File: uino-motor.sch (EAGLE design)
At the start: 31 parts, among them J1 CON_TERMINAL_BLOCK_02-5MM, J2 CON_TERMINAL_BLOCK_02-5MM, J3 CON_TERMINAL_BLOCK_02-5MM, Q1 P-FET, U1 74*1G57, U2 74*1G57

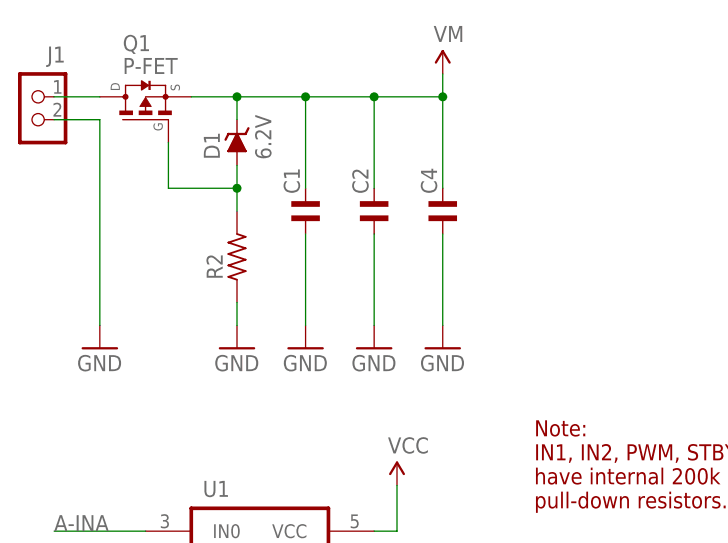
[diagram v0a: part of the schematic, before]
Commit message: Parts placed and major routing completed.
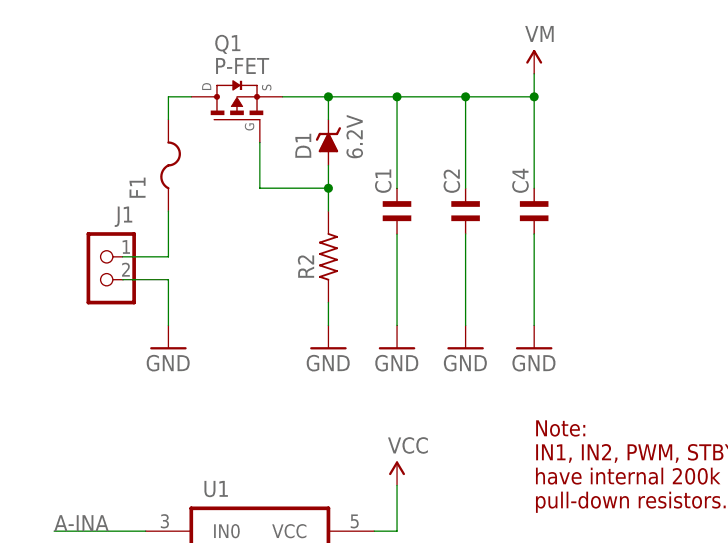
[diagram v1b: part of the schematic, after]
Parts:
- added F1: (no value), adi-misc:FUSE_PTC-TH
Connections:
- net N$10 renamed A01
- net N$11 renamed B01
- net N$12 renamed A02
- net N$13 renamed B02
- removed net N$8: J1.1, Q1.D
- new net N$5: F1.1, J1.1
- new net N$7: F1.2, Q1.D
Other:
- moved on the sheet: C1, C2, C4, D1, J1, Q1, R2
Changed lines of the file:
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@@
 <part name="R5" library="rc-master-smd" deviceset="R_" device="0805MP"/>
 <part name="GND15" library="SparkFun-Aesthetics" deviceset="GND" device=""/>
+<part name="F1" library="adi-misc" deviceset="FUSE_PTC" device="-TH"/>
 </parts>
 <sheets>
@@
 <instance part="J2" gate="CON" x="132.08" y="81.28" rot="MR180"/>
 <instance part="J3" gate="CON" x="132.08" y="60.96" rot="MR180"/>
-<instance part="J1" gate="CON" x="5.08" y="152.4" rot="MR0"/>
+<instance part="J1" gate="CON" x="12.7" y="134.62" rot="MR0"/>
 <instance part="GND8" gate="1" x="121.92" y="50.8"/>
 <instance part="GND3" gate="1" x="83.82" y="50.8"/>
@@
 <instance part="R1" gate="G$1" x="71.12" y="73.66"/>
 <instance part="SUPPLY3" gate="G$1" x="60.96" y="91.44"/>
-<instance part="Q1" gate="G$1" x="15.24" y="152.4" smashed="yes" rot="R90">
-<attribute name="VALUE" x="12.7" y="154.94" size="1.778" layer="96"/>
-<attribute name="NAME" x="12.7" y="157.48" size="1.778" layer="95"/>
+<instance part="Q1" gate="G$1" x="25.4" y="152.4" smashed="yes" rot="R90">
+<attribute name="VALUE" x="22.86" y="154.94" size="1.778" layer="96"/>
+<attribute name="NAME" x="22.86" y="157.48" size="1.778" layer="95"/>
 </instance>
-<instance part="D1" gate="G$1" x="25.4" y="147.32" rot="R90"/>
-<instance part="R2" gate="G$1" x="25.4" y="134.62" rot="R90"/>
-<instance part="GND5" gate="1" x="25.4" y="124.46"/>
-<instance part="SUPPLY6" gate="VDD" x="48.26" y="154.94"/>
-<instance part="C1" gate="G$1" x="33.02" y="139.7" rot="R90"/>
-<instance part="C2" gate="G$1" x="40.64" y="139.7" rot="R90"/>
-<instance part="GND6" gate="1" x="33.02" y="124.46"/>
-<instance part="GND7" gate="1" x="40.64" y="124.46"/>
-<instance part="GND4" gate="1" x="10.16" y="124.46"/>
+<instance part="D1" gate="G$1" x="35.56" y="147.32" rot="R90"/>
+<instance part="R2" gate="G$1" x="35.56" y="134.62" rot="R90"/>
+<instance part="GND5" gate="1" x="35.56" y="124.46"/>
+<instance part="SUPPLY6" gate="VDD" x="58.42" y="154.94"/>
+<instance part="C1" gate="G$1" x="43.18" y="139.7" rot="R90"/>
+<instance part="C2" gate="G$1" x="50.8" y="139.7" rot="R90"/>
+<instance part="GND6" gate="1" x="43.18" y="124.46"/>
+<instance part="GND7" gate="1" x="50.8" y="124.46"/>
+<instance part="GND4" gate="1" x="17.78" y="124.46"/>
 <instance part="JP2" gate="G$1" x="157.48" y="114.3"/>
 <instance part="JP3" gate="G$1" x="157.48" y="106.68"/>
@@
 <instance part="GND11" gate="1" x="60.96" y="50.8"/>
 <instance part="U$1" gate="G$1" x="101.6" y="73.66" rot="MR0"/>
-<instance part="C4" gate="G$1" x="48.26" y="139.7" rot="R90"/>
-<instance part="GND12" gate="1" x="48.26" y="124.46"/>
+<instance part="C4" gate="G$1" x="58.42" y="139.7" rot="R90"/>
+<instance part="GND12" gate="1" x="58.42" y="124.46"/>
 <instance part="R3" gate="G$1" x="99.06" y="116.84" rot="R90"/>
 <instance part="GND13" gate="1" x="99.06" y="106.68"/>
@@
 <instance part="R5" gate="G$1" x="129.54" y="116.84" rot="R90"/>
 <instance part="GND15" gate="1" x="129.54" y="106.68"/>
+<instance part="F1" gate="G$1" x="20.32" y="144.78" rot="R90"/>
 </instances>
 <busses>
@@
 <pinref part="C2" gate="G$1" pin="1"/>
 <pinref part="GND7" gate="1" pin="GND"/>
-<wire x1="40.64" y1="137.16" x2="40.64" y2="127" width="0.1524" layer="91"/>
+<wire x1="50.8" y1="137.16" x2="50.8" y2="127" width="0.1524" layer="91"/>
 </segment>
 <segment>
 <pinref part="C1" gate="G$1" pin="1"/>
 <pinref part="GND6" gate="1" pin="GND"/>
-<wire x1="33.02" y1="137.16" x2="33.02" y2="127" width="0.1524" layer="91"/>
-</segment>
-<segment>
-<pinref part="J1" gate="CON" pin="2"/>
-<pinref part="GND4" gate="1" pin="GND"/>
-<wire x1="5.08" y1="149.86" x2="10.16" y2="149.86" width="0.1524" layer="91"/>
-<wire x1="10.16" y1="149.86" x2="10.16" y2="127" width="0.1524" layer="91"/>
+<wire x1="43.18" y1="137.16" x2="43.18" y2="127" width="0.1524" layer="91"/>
 </segment>
 <segment>
 <pinref part="R2" gate="G$1" pin="1"/>
 <pinref part="GND5" gate="1" pin="GND"/>
-<wire x1="25.4" y1="129.54" x2="25.4" y2="127" width="0.1524" layer="91"/>
+<wire x1="35.56" y1="129.54" x2="35.56" y2="127" width="0.1524" layer="91"/>
 </segment>
 <segment>
@@
 <pinref part="C4" gate="G$1" pin="1"/>
 <pinref part="GND12" gate="1" pin="GND"/>
-<wire x1="48.26" y1="137.16" x2="48.26" y2="127" width="0.1524" layer="91"/>
+<wire x1="58.42" y1="137.16" x2="58.42" y2="127" width="0.1524" layer="91"/>
 </segment>
 <segment>
@@
 <pinref part="GND15" gate="1" pin="GND"/>
 <wire x1="129.54" y1="111.76" x2="129.54" y2="109.22" width="0.1524" layer="91"/>
+</segment>
+<segment>
+<pinref part="J1" gate="CON" pin="2"/>
+<pinref part="GND4" gate="1" pin="GND"/>
+<wire x1="12.7" y1="132.08" x2="17.78" y2="132.08" width="0.1524" layer="91"/>
+<wire x1="17.78" y1="132.08" x2="17.78" y2="127" width="0.1524" layer="91"/>
 </segment>
 </net>
@@
 <pinref part="C2" gate="G$1" pin="2"/>
 <pinref part="Q1" gate="G$1" pin="S"/>
-<wire x1="40.64" y1="152.4" x2="40.64" y2="142.24" width="0.1524" layer="91"/>
-<wire x1="20.32" y1="152.4" x2="25.4" y2="152.4" width="0.1524" layer="91"/>
-<junction x="40.64" y="152.4"/>
+<wire x1="50.8" y1="152.4" x2="50.8" y2="142.24" width="0.1524" layer="91"/>
+<wire x1="30.48" y1="152.4" x2="35.56" y2="152.4" width="0.1524" layer="91"/>
+<junction x="50.8" y="152.4"/>
 <pinref part="D1" gate="G$1" pin="C"/>
-<wire x1="25.4" y1="152.4" x2="33.02" y2="152.4" width="0.1524" layer="91"/>
-<wire x1="33.02" y1="152.4" x2="40.64" y2="152.4" width="0.1524" layer="91"/>
-<wire x1="25.4" y1="149.86" x2="25.4" y2="152.4" width="0.1524" layer="91"/>
-<junction x="25.4" y="152.4"/>
+<wire x1="35.56" y1="152.4" x2="43.18" y2="152.4" width="0.1524" layer="91"/>
+<wire x1="43.18" y1="152.4" x2="50.8" y2="152.4" width="0.1524" layer="91"/>
+<wire x1="35.56" y1="149.86" x2="35.56" y2="152.4" width="0.1524" layer="91"/>
+<junction x="35.56" y="152.4"/>
 <pinref part="C1" gate="G$1" pin="2"/>
-<wire x1="33.02" y1="142.24" x2="33.02" y2="152.4" width="0.1524" layer="91"/>
-<junction x="33.02" y="152.4"/>
+<wire x1="43.18" y1="142.24" x2="43.18" y2="152.4" width="0.1524" layer="91"/>
+<junction x="43.18" y="152.4"/>
 <pinref part="C4" gate="G$1" pin="2"/>
-<wire x1="40.64" y1="152.4" x2="48.26" y2="152.4" width="0.1524" layer="91"/>
-<wire x1="48.26" y1="152.4" x2="48.26" y2="142.24" width="0.1524" layer="91"/>
+<wire x1="50.8" y1="152.4" x2="58.42" y2="152.4" width="0.1524" layer="91"/>
+<wire x1="58.42" y1="152.4" x2="58.42" y2="142.24" width="0.1524" layer="91"/>
 <pinref part="SUPPLY6" gate="VDD" pin="VDD"/>
-<wire x1="48.26" y1="154.94" x2="48.26" y2="152.4" width="0.1524" layer="91"/>
-<junction x="48.26" y="152.4"/>
+<wire x1="58.42" y1="154.94" x2="58.42" y2="152.4" width="0.1524" layer="91"/>
+<junction x="58.42" y="152.4"/>
 </segment>
 </net>
@@
 <segment>
 <pinref part="D1" gate="G$1" pin="A"/>
-<wire x1="25.4" y1="144.78" x2="25.4" y2="142.24" width="0.1524" layer="91"/>
+<wire x1="35.56" y1="144.78" x2="35.56" y2="142.24" width="0.1524" layer="91"/>
 <pinref part="Q1" gate="G$1" pin="G"/>
-<wire x1="17.78" y1="147.32" x2="17.78" y2="142.24" width="0.1524" layer="91"/>
-<wire x1="17.78" y1="142.24" x2="25.4" y2="142.24" width="0.1524" layer="91"/>
+<wire x1="27.94" y1="147.32" x2="27.94" y2="142.24" width="0.1524" layer="91"/>
+<wire x1="27.94" y1="142.24" x2="35.56" y2="142.24" width="0.1524" layer="91"/>
 <pinref part="R2" gate="G$1" pin="2"/>
-<wire x1="25.4" y1="139.7" x2="25.4" y2="142.24" width="0.1524" layer="91"/>
-<junction x="25.4" y="142.24"/>
-</segment>
-</net>
-<net name="N$8" class="0">
-<segment>
-<pinref part="J1" gate="CON" pin="1"/>
-<pinref part="Q1" gate="G$1" pin="D"/>
-<wire x1="5.08" y1="152.4" x2="10.16" y2="152.4" width="0.1524" layer="91"/>
+<wire x1="35.56" y1="139.7" x2="35.56" y2="142.24" width="0.1524" layer="91"/>
+<junction x="35.56" y="142.24"/>
 </segment>
 </net>
@@
 </segment>
 </net>
-<net name="N$10" class="0">
+<net name="A01" class="0">
 <segment>
 <pinref part="U$1" gate="G$1" pin="A01@1"/>
@@
 </segment>
 </net>
-<net name="N$11" class="0">
+<net name="B01" class="0">
 <segment>
 <pinref part="U$1" gate="G$1" pin="B01@12"/>
@@
 </segment>
 </net>
-<net name="N$12" class="0">
+<net name="A02" class="0">
 <segment>
 <pinref part="U$1" gate="G$1" pin="A02@6"/>
@@
 </segment>
 </net>
-<net name="N$13" class="0">
+<net name="B02" class="0">
 <segment>
 <pinref part="U$1" gate="G$1" pin="B02@7"/>
@@
 </segment>
 </net>
+<net name="N$5" class="0">
+<segment>
+<pinref part="J1" gate="CON" pin="1"/>
+<pinref part="F1" gate="G$1" pin="1"/>
+<wire x1="12.7" y1="134.62" x2="17.78" y2="134.62" width="0.1524" layer="91"/>
+<wire x1="17.78" y1="134.62" x2="17.78" y2="139.7" width="0.1524" layer="91"/>
+</segment>
+</net>
+<net name="N$7" class="0">
+<segment>
+<pinref part="F1" gate="G$1" pin="2"/>
+<wire x1="17.78" y1="149.86" x2="17.78" y2="152.4" width="0.1524" layer="91"/>
+<pinref part="Q1" gate="G$1" pin="D"/>
+<wire x1="17.78" y1="152.4" x2="20.32" y2="152.4" width="0.1524" layer="91"/>
+</segment>
+</net>
